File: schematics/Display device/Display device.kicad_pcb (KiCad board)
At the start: 2 copper layers, 57.5 x 44.5 mm, 11 parts, among them J1 stepper motor, SW1 SW_Push, U1 XIAO ESP32C3

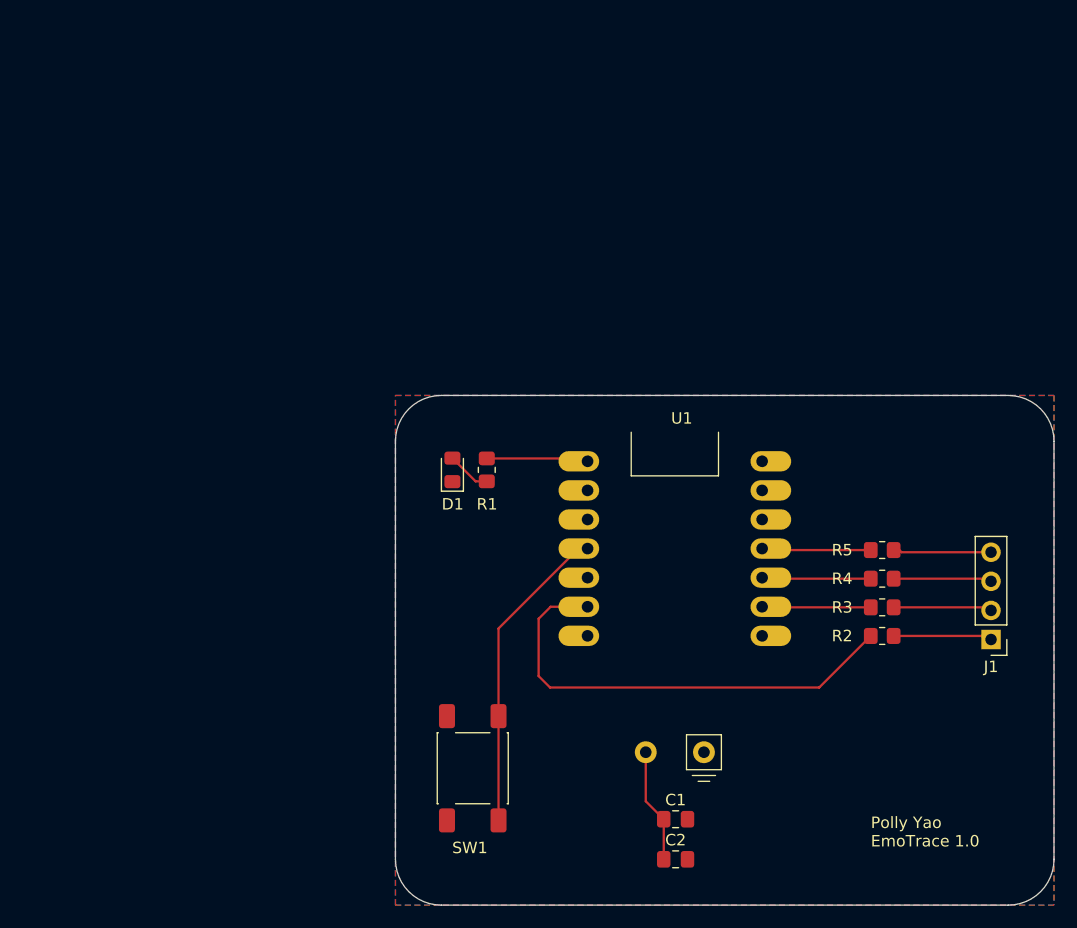
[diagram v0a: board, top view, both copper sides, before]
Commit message: kicad update
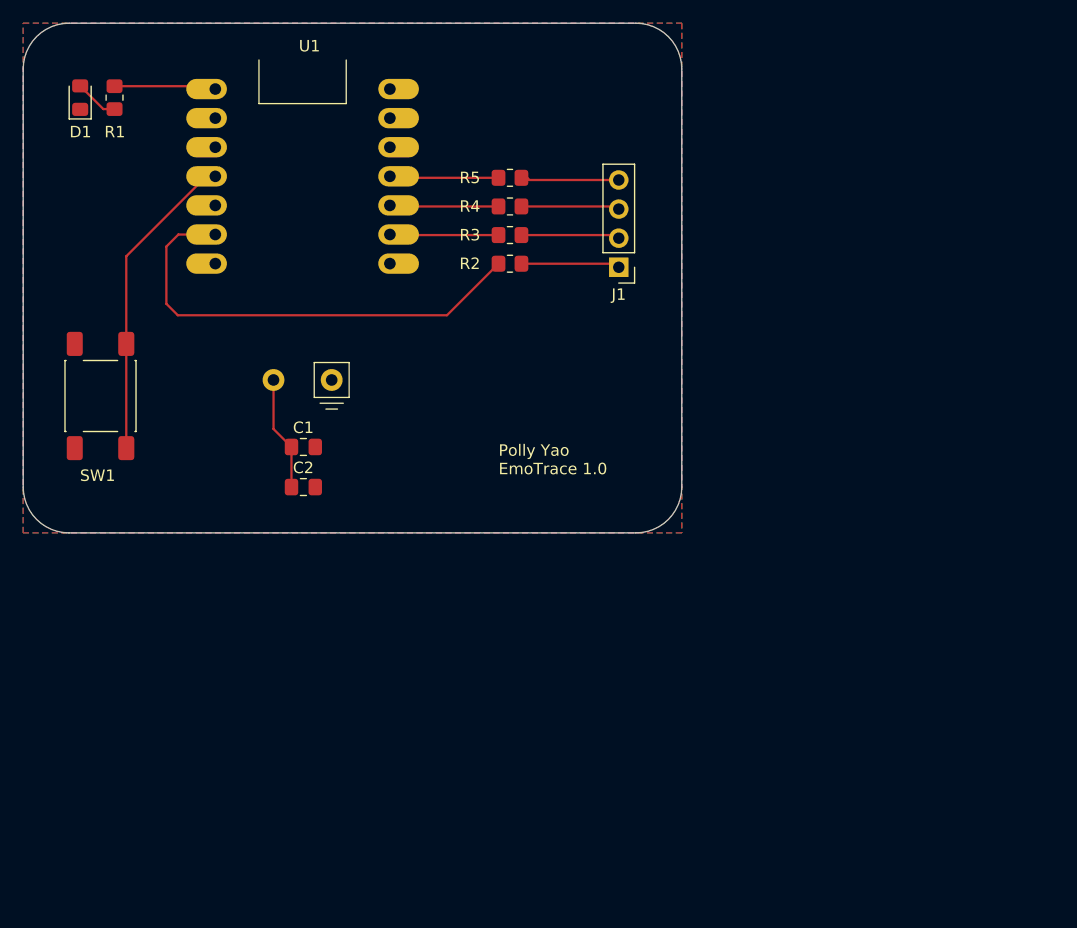
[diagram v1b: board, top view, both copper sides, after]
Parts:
- moved U1 46.0 mm to (100.9, 56.4)
- moved C1 46.0 mm to (101.0, 80.0)
- moved C2 46.0 mm to (101.0, 83.5)
- moved D1 46.0 mm to (81.5, 49.5)
- moved J1 46.0 mm to (128.5, 64.3)
- moved R1 46.0 mm to (84.5, 49.5)
- moved R2 46.0 mm to (119.0, 64.0)
- moved R3 46.0 mm to (119.0, 61.5)
- moved R4 46.0 mm to (119.0, 59.0)
- moved R5 46.0 mm to (119.0, 56.5)
- moved SW1 46.0 mm to (83.2, 75.5)
